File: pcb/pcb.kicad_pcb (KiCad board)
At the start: 4 copper layers, 32 x 39 mm, 88 parts, among them U1 JM20330, U2 SM2258XT, U3 FlashBGA152, U4 Conn_41PIN, U5 SY8008, U6 SY8008, U7 TX4314, Y1 25MHz, Y2 50MHz

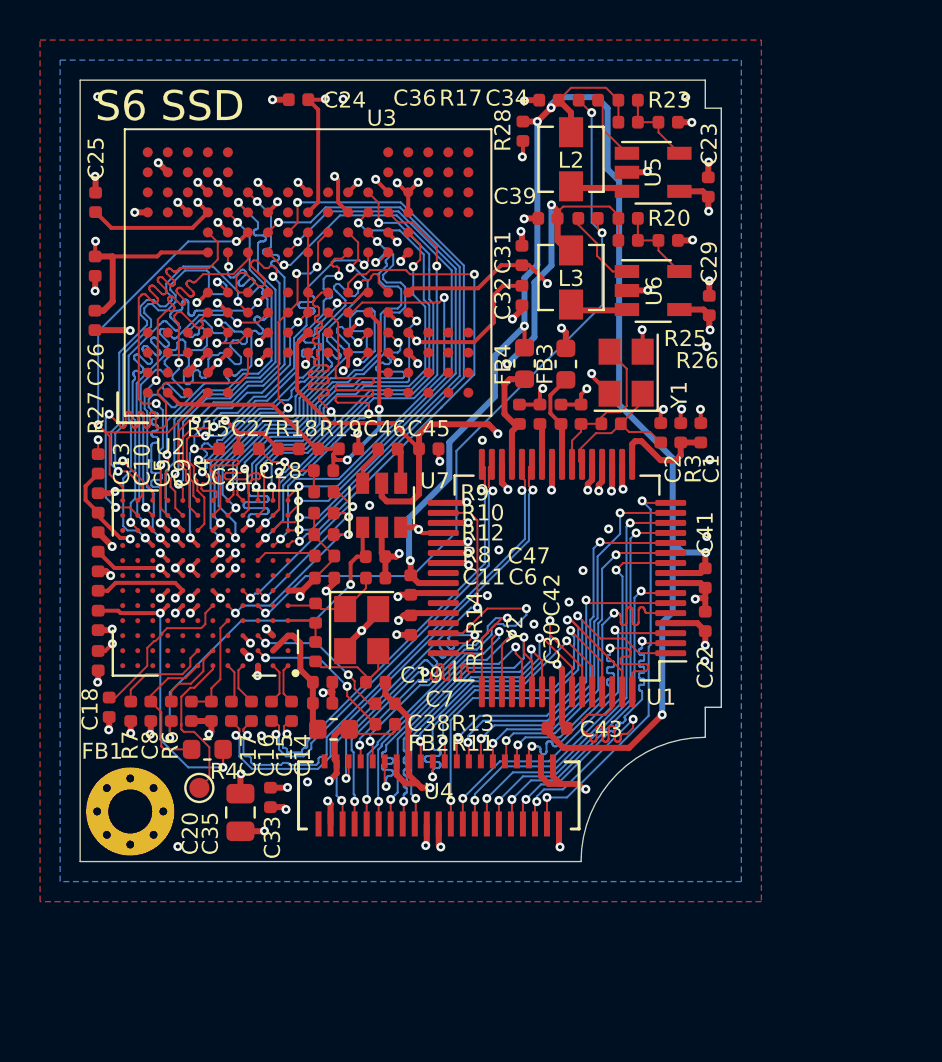
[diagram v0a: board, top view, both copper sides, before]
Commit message: Upgrade to 5.99, clean up
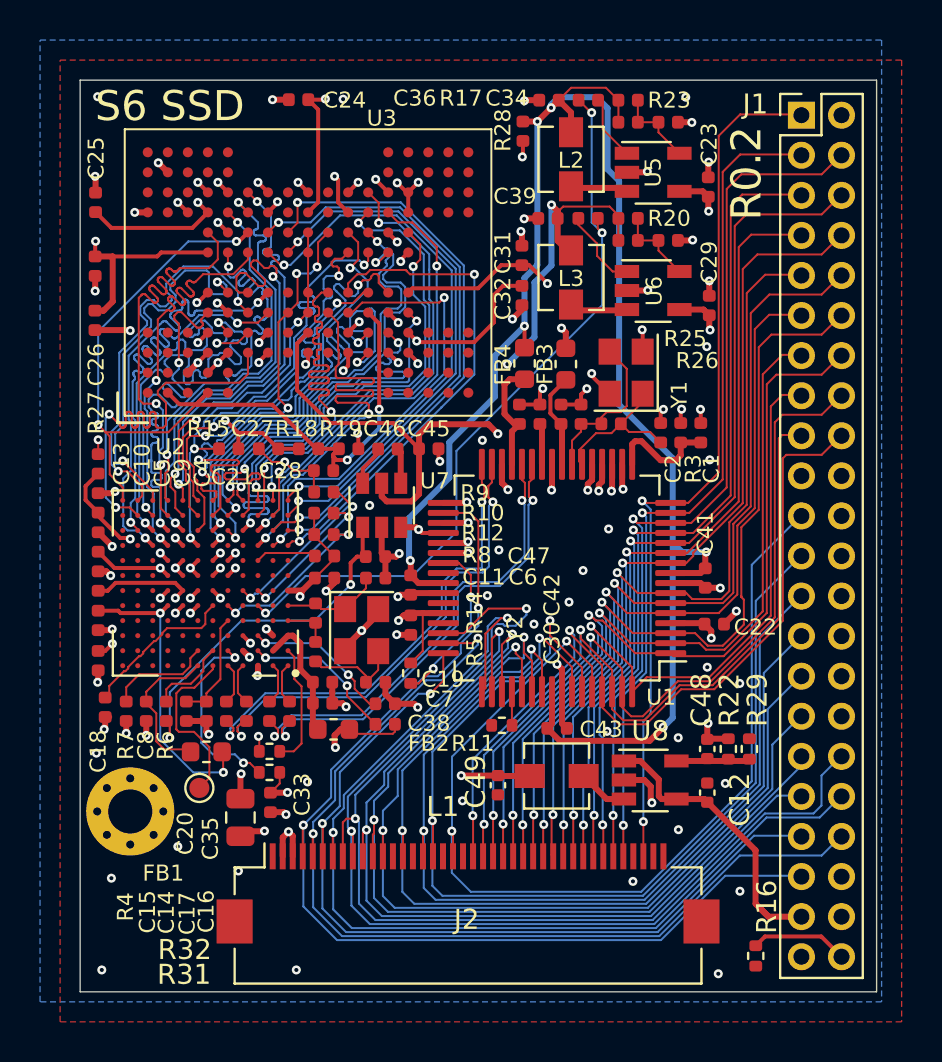
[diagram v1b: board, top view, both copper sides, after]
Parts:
- removed U4: Conn_41PIN, Footprints:FH35C-41S-0.3SHW
- added C12: 470nF, Capacitor_SMD:C_0402_1005Metric, F.Cu at (161.3, 126.6)
- added C48: 22pF, Capacitor_SMD:C_0402_1005Metric, F.Cu at (161.3, 124.4)
- added C49: 4.7uF, Capacitor_SMD:C_0402_1005Metric, F.Cu at (150.8, 126.2)
- added J1: Conn_02x22_Odd_Even, Connector_PinHeader_2.00mm:PinHeader_2x22_P2.00mm_Vertical, F.Cu at (166.0, 92.8)
- added J2: Conn_01x40_MountingPin, Connector_FFC-FPC:Hirose_FH12-40S-0.5SH_1x40-1MP_P0.50mm_Horizontal, F.Cu at (149.4, 131.6)
- added L1: 2.2uH, Inductor_SMD:L_Vishay_IHLP-1212, F.Cu at (153.8, 125.7)
- added R16: 10K, Resistor_SMD:R_0402_1005Metric, F.Cu at (163.7, 134.7)
- added R21: 10K, Resistor_SMD:R_0402_1005Metric, F.Cu at (151.1, 123.2)
- added R22: 46.4K, Resistor_SMD:R_0402_1005Metric, F.Cu at (162.3, 124.4)
- added R29: 10K, Resistor_SMD:R_0402_1005Metric, F.Cu at (163.4, 124.4)
- added R30: 10K, Resistor_SMD:R_0402_1005Metric, F.Cu at (146.5, 120.6)
- added R31: 10K, Resistor_SMD:R_0402_1005Metric, F.Cu at (139.4, 125.5)
- added R32: 200/1%, Resistor_SMD:R_0402_1005Metric, F.Cu at (139.4, 124.5)
- added U8: SY8008, Package_TO_SOT_SMD:TSOT-23-5, F.Cu at (158.4, 125.9)
- R12: value 10K -> NC
- R7: value 10K -> 0
- moved C14 2.25 mm to (138.3, 122.5)
- moved C15 2.25 mm to (137.3, 122.5)
- moved C16 1.90 mm to (140.4, 122.5)
- moved C17 1.90 mm to (139.4, 122.5)
- moved C22 0.47 mm to (161.7, 118.2), turned to 180 degrees
- moved C20 0.25 mm to (135.3, 122.5)
- moved C33 0.25 mm to (139.5, 127.0)
- moved C35 0.25 mm to (138.0, 127.8)
- moved R4 0.25 mm to (136.3, 122.5)
- moved R6 0.25 mm to (134.3, 122.5)
- moved C8 0.22 mm to (133.3, 122.5)
- moved R7 0.22 mm to (132.3, 122.5)
- moved C18 0.20 mm to (131.2, 122.3)
- moved FB1 0.13 mm to (136.3, 124.5)
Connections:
- U1 pad 27: Net-(C17-Pad1) -> Net-(C16-Pad1)
- U1 pad 28: Net-(C16-Pad1) -> Net-(C17-Pad1)
- U1 pad 31: Net-(C15-Pad1) -> Net-(C14-Pad1)
- U1 pad 32: Net-(C14-Pad1) -> Net-(C15-Pad1)
- U1 pad 39: GND -> Net-(R30-Pad2)
- U1 pad 40: (no net) -> unconnected-(U1-Pad40)
- U1 pad 43: (no net) -> unconnected-(U1-Pad43)
- U1 pad 45: (no net) -> unconnected-(U1-Pad45)
- U1 pad 52: (no net) -> Net-(R21-Pad1)
- U2 pad A1: Net-(C14-Pad2) -> Net-(C16-Pad2)
- U2 pad A10: (no net) -> unconnected-(U2-PadA10)
- U2 pad A11: (no net) -> unconnected-(U2-PadA11)
- U2 pad A12: (no net) -> unconnected-(U2-PadA12)
- U2 pad A2: Net-(C15-Pad2) -> Net-(C17-Pad2)
- U2 pad A4: Net-(C16-Pad2) -> Net-(C14-Pad2)
- U2 pad A5: Net-(C17-Pad2) -> Net-(C15-Pad2)
- U2 pad A8: (no net) -> unconnected-(U2-PadA8)
- U2 pad A9: (no net) -> unconnected-(U2-PadA9)
- U2 pad B1: (no net) -> Net-(R32-Pad1)
- U2 pad B10: (no net) -> unconnected-(U2-PadB10)
- U2 pad B11: (no net) -> unconnected-(U2-PadB11)
- U2 pad B12: (no net) -> unconnected-(U2-PadB12)
- U2 pad B5: (no net) -> Net-(R31-Pad1)
- U2 pad B8: (no net) -> unconnected-(U2-PadB8)
- U2 pad B9: (no net) -> unconnected-(U2-PadB9)
- U2 pad C10: (no net) -> unconnected-(U2-PadC10)
- U2 pad C11: (no net) -> unconnected-(U2-PadC11)
- U2 pad C12: (no net) -> unconnected-(U2-PadC12)
- U2 pad C5: (no net) -> unconnected-(U2-PadC5)
- U2 pad C6: (no net) -> unconnected-(U2-PadC6)
- U2 pad C7: (no net) -> unconnected-(U2-PadC7)
- U2 pad C8: (no net) -> unconnected-(U2-PadC8)
- U2 pad C9: (no net) -> unconnected-(U2-PadC9)
- U2 pad D10: (no net) -> unconnected-(U2-PadD10)
- U2 pad D11: (no net) -> unconnected-(U2-PadD11)
- U2 pad D12: (no net) -> unconnected-(U2-PadD12)
- U2 pad D2: (no net) -> unconnected-(U2-PadD2)
- U2 pad D3: (no net) -> unconnected-(U2-PadD3)
- U2 pad D4: (no net) -> unconnected-(U2-PadD4)
- U2 pad D6: (no net) -> unconnected-(U2-PadD6)
- U2 pad D7: (no net) -> unconnected-(U2-PadD7)
- U2 pad D8: (no net) -> unconnected-(U2-PadD8)
- U2 pad D9: (no net) -> unconnected-(U2-PadD9)
- U2 pad E10: (no net) -> unconnected-(U2-PadE10)
- U2 pad E11: (no net) -> unconnected-(U2-PadE11)
- U2 pad E12: (no net) -> unconnected-(U2-PadE12)
- U2 pad E2: (no net) -> unconnected-(U2-PadE2)
- U2 pad E4: (no net) -> unconnected-(U2-PadE4)
- U2 pad F10: (no net) -> unconnected-(U2-PadF10)
- U2 pad F11: (no net) -> unconnected-(U2-PadF11)
- U2 pad F12: (no net) -> unconnected-(U2-PadF12)
- U2 pad F2: (no net) -> unconnected-(U2-PadF2)
- U2 pad F5: (no net) -> unconnected-(U2-PadF5)
- U2 pad G1: (no net) -> unconnected-(U2-PadG1)
- U2 pad G10: (no net) -> unconnected-(U2-PadG10)
- U2 pad G11: (no net) -> unconnected-(U2-PadG11)
- U2 pad G12: (no net) -> unconnected-(U2-PadG12)
- U2 pad G2: (no net) -> unconnected-(U2-PadG2)
- U2 pad G3: (no net) -> unconnected-(U2-PadG3)
- U2 pad G4: (no net) -> unconnected-(U2-PadG4)
- U2 pad H1: (no net) -> unconnected-(U2-PadH1)
- U2 pad H10: (no net) -> unconnected-(U2-PadH10)
- U2 pad H11: (no net) -> unconnected-(U2-PadH11)
- U2 pad H12: (no net) -> unconnected-(U2-PadH12)
- U2 pad H2: (no net) -> unconnected-(U2-PadH2)
- U2 pad H4: (no net) -> unconnected-(U2-PadH4)
- U2 pad J11: (no net) -> unconnected-(U2-PadJ11)
- U2 pad J12: (no net) -> unconnected-(U2-PadJ12)
- U2 pad J4: (no net) -> unconnected-(U2-PadJ4)
- U2 pad J5: (no net) -> unconnected-(U2-PadJ5)
- U2 pad K12: (no net) -> unconnected-(U2-PadK12)
- U2 pad L12: (no net) -> unconnected-(U2-PadL12)
- U3 pad A1: Net-(U3-PadA1) -> unconnected-(U3-PadA1)
- U3 pad A11: Net-(U3-PadA11) -> unconnected-(U3-PadA11)
- U3 pad A12: Net-(U3-PadA12) -> unconnected-(U3-PadA12)
- U3 pad A13: Net-(U3-PadA13) -> unconnected-(U3-PadA13)
- U3 pad A2: Net-(U3-PadA2) -> unconnected-(U3-PadA2)
- U3 pad A3: Net-(U3-PadA3) -> unconnected-(U3-PadA3)
- U3 pad A4: Net-(U3-PadA4) -> unconnected-(U3-PadA4)
- U3 pad B10: Net-(U3-PadB10) -> unconnected-(U3-PadB10)
- U3 pad B11: Net-(U3-PadB11) -> unconnected-(U3-PadB11)
- U3 pad B13: Net-(U3-PadB13) -> unconnected-(U3-PadB13)
- U3 pad B2: Net-(U3-PadB2) -> unconnected-(U3-PadB2)
- U3 pad B3: Net-(U3-PadB3) -> unconnected-(U3-PadB3)
- U3 pad B4: Net-(U3-PadB4) -> unconnected-(U3-PadB4)
- U3 pad C1: Net-(U3-PadC1) -> unconnected-(U3-PadC1)
- U3 pad C11: Net-(U3-PadC11) -> unconnected-(U3-PadC11)
- U3 pad C12: Net-(U3-PadC12) -> unconnected-(U3-PadC12)
- U3 pad C13: Net-(U3-PadC13) -> unconnected-(U3-PadC13)
- U3 pad C3: Net-(U3-PadC3) -> unconnected-(U3-PadC3)
- U3 pad C4: Net-(U3-PadC4) -> unconnected-(U3-PadC4)
- U3 pad D12: Net-(U3-PadD12) -> unconnected-(U3-PadD12)
- U3 pad D13: Net-(U3-PadD13) -> unconnected-(U3-PadD13)
- U3 pad E1: Net-(U3-PadE1) -> unconnected-(U3-PadE1)
- U3 pad E12: Net-(U3-PadE12) -> unconnected-(U3-PadE12)
- U3 pad E13: Net-(U3-PadE13) -> unconnected-(U3-PadE13)
- U3 pad E2: Net-(U3-PadE2) -> unconnected-(U3-PadE2)
- U3 pad H10: Net-(U3-PadH10) -> unconnected-(U3-PadH10)
- U3 pad H11: Net-(U3-PadH11) -> unconnected-(U3-PadH11)
- U3 pad H3: Net-(U3-PadH3) -> unconnected-(U3-PadH3)
- U3 pad H4: Net-(U3-PadH4) -> unconnected-(U3-PadH4)
- U3 pad H6: Net-(U3-PadH6) -> unconnected-(U3-PadH6)
- U3 pad K10: Net-(U3-PadK10) -> unconnected-(U3-PadK10)
- U3 pad K11: Net-(U3-PadK11) -> unconnected-(U3-PadK11)
- U3 pad K3: Net-(U3-PadK3) -> unconnected-(U3-PadK3)
- U3 pad K4: Net-(U3-PadK4) -> unconnected-(U3-PadK4)
- U3 pad K8: Net-(U3-PadK8) -> unconnected-(U3-PadK8)
- U3 pad N1: Net-(U3-PadN1) -> unconnected-(U3-PadN1)
- U3 pad N12: Net-(U3-PadN12) -> unconnected-(U3-PadN12)
- U3 pad N13: Net-(U3-PadN13) -> unconnected-(U3-PadN13)
- U3 pad N2: Net-(U3-PadN2) -> unconnected-(U3-PadN2)
- U3 pad R1: Net-(U3-PadR1) -> unconnected-(U3-PadR1)
- U3 pad R10: Net-(U3-PadR10) -> unconnected-(U3-PadR10)
- U3 pad R11: Net-(U3-PadR11) -> unconnected-(U3-PadR11)
- U3 pad R12: Net-(U3-PadR12) -> unconnected-(U3-PadR12)
- U3 pad R13: Net-(U3-PadR13) -> unconnected-(U3-PadR13)
- U3 pad R2: Net-(U3-PadR2) -> unconnected-(U3-PadR2)
- U3 pad R3: Net-(U3-PadR3) -> unconnected-(U3-PadR3)
- U3 pad R4: Net-(U3-PadR4) -> unconnected-(U3-PadR4)
- U3 pad T1: Net-(U3-PadT1) -> unconnected-(U3-PadT1)
- U3 pad T10: Net-(U3-PadT10) -> unconnected-(U3-PadT10)
- U3 pad T11: Net-(U3-PadT11) -> unconnected-(U3-PadT11)
- U3 pad T12: Net-(U3-PadT12) -> unconnected-(U3-PadT12)
- U3 pad T13: Net-(U3-PadT13) -> unconnected-(U3-PadT13)
- U3 pad T2: Net-(U3-PadT2) -> unconnected-(U3-PadT2)
- U3 pad T3: Net-(U3-PadT3) -> unconnected-(U3-PadT3)
- U3 pad T4: Net-(U3-PadT4) -> unconnected-(U3-PadT4)
- U3 pad U1: Net-(U3-PadU1) -> unconnected-(U3-PadU1)
- U3 pad U10: Net-(U3-PadU10) -> unconnected-(U3-PadU10)
- U3 pad U11: Net-(U3-PadU11) -> unconnected-(U3-PadU11)
- U3 pad U12: Net-(U3-PadU12) -> unconnected-(U3-PadU12)
- U3 pad U13: Net-(U3-PadU13) -> unconnected-(U3-PadU13)
- U3 pad U2: Net-(U3-PadU2) -> unconnected-(U3-PadU2)
- U3 pad U3: Net-(U3-PadU3) -> unconnected-(U3-PadU3)
- U3 pad U4: Net-(U3-PadU4) -> unconnected-(U3-PadU4)
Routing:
- net /IDE_IOW: track 15.4 -> 53.2 mm
- net /IDE_PDIAG: track 16.9 -> 54.4 mm
- net /IDE_A2: track 15.6 -> 52.6 mm
- net /IDE_DMARQ: track 16.7 -> 50.2 mm
- net /IDE_DASP: track 20.2 -> 53.6 mm
- net /IDE_CS1: track 16.0 -> 49.3 mm
- net /IDE_IOR: track 16.9 -> 49.9 mm
- net /IDE_DMACK: track 16.3 -> 48.7 mm
- net /IDE_IORDY: track 15.9 -> 48.0 mm
- net /IDE_A0: track 16.0 -> 47.2 mm
- net /IDE_INTRQ: track 15.9 -> 46.7 mm
- net /IDE_A1: track 16.0 -> 46.4 mm
- net /IDE_D15: track 15.3 -> 41.0 mm
- net /IDE_CS0: track 18.0 -> 43.6 mm
- net /IDE_D12: track 17.2 -> 42.0 mm
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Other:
- board size 32 x 39 mm -> 39.8 x 45.5 mm
- net class Default removed
- rule pad_to_mask_clearance: 0.05 -> 0
- board text added: "R0.2"
- board text added: "S6 SSD Copyright 2021 W.Z."
- board text removed: "S6 SSD Copyright 2020 W.Z."

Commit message: Rev 0.3
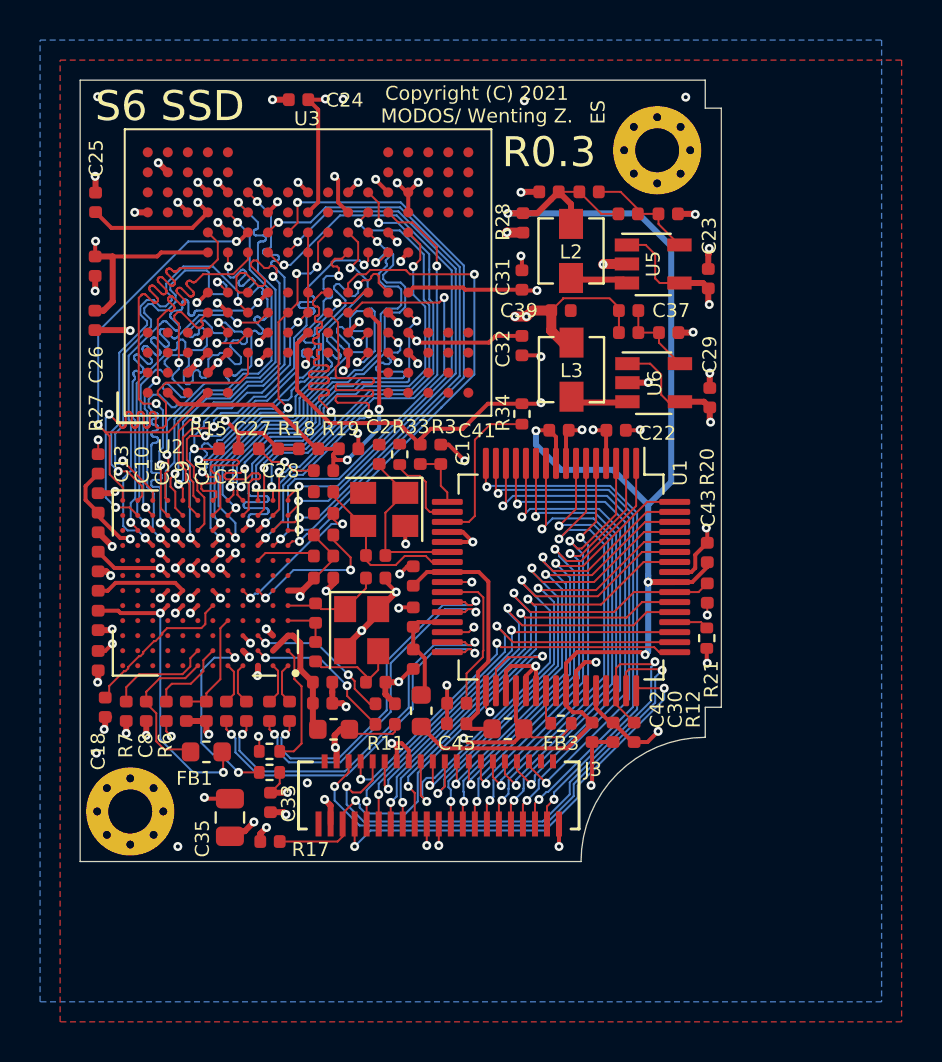
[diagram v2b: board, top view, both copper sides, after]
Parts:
- removed C12: 470nF, Capacitor_SMD:C_0402_1005Metric
- removed C47: 10uF, Capacitor_SMD:C_0402_1005Metric
- removed C48: 22pF, Capacitor_SMD:C_0402_1005Metric
- removed C49: 4.7uF, Capacitor_SMD:C_0402_1005Metric
- removed J1: Conn_02x22_Odd_Even, Connector_PinHeader_2.00mm:PinHeader_2x22_P2.00mm_Vertical
- removed J2: Conn_01x40_MountingPin, Connector_FFC-FPC:Hirose_FH12-40S-0.5SH_1x40-1MP_P0.50mm_Horizontal
- removed L1: 2.2uH, Inductor_SMD:L_Vishay_IHLP-1212
- removed R16, R29: 10K, Resistor_SMD:R_0402_1005Metric
- removed R22: 46.4K, Resistor_SMD:R_0402_1005Metric
- removed TP7: TestPoint, TestPoint:TestPoint_Pad_D1.0mm
- removed U7: TX4314, Package_TO_SOT_SMD:SOT-23-6
- removed U8: SY8008, Package_TO_SOT_SMD:TSOT-23-5
- added H2: MountingHole_Pad, MountingHole:MountingHole_2.2mm_M2_Pad_Via, F.Cu at (158.8, 94.5)
- added J3: S6, Footprints:FH35C-41S-0.3SHW, F.Cu at (147.9, 126.7)
- added R33: 0, Resistor_SMD:R_0402_1005Metric, F.Cu at (145.9, 109.7)
- added R34: 0, Resistor_SMD:R_0402_1005Metric, F.Cu at (152.1, 107.7)
- C31, C32, C33, C36, C38, C39: value 4.7uF -> 10uF
- H1: value MountingHole -> MountingHole_Pad
- R12, R13: value NC -> 10K
- R6: value 5.1K -> 2K
- moved R17 40.3 mm to (139.5, 129.0), turned to 0 degrees
- moved R20 19.6 mm to (161.3, 116.6), turned to 90 degrees
- moved FB3 18.4 mm to (151.3, 123.4), turned to 0 degrees
- moved R12 18.4 mm to (157.7, 123.5), turned to 90 degrees
- moved FB4 18.1 mm to (147.0, 122.5), turned to -90 degrees
- moved R1 15.0 mm to (148.8, 122.1), turned to 0 degrees
- moved C2 14.1 mm to (144.9, 109.7)
- moved Y1 13.9 mm to (145.2, 112.4), turned to 180 degrees
- moved C45 13.8 mm to (148.8, 123.1), turned to 0 degrees
- moved R2 13.5 mm to (144.8, 114.7)
- moved C3 13.4 mm to (142.2, 111.5), turned to 180 degrees
- moved R3 13.0 mm to (147.0, 109.7)
- moved C1 13.0 mm to (148.0, 109.7)
- moved C42 11.7 mm to (155.6, 123.5)
- moved C43 11.5 mm to (161.3, 114.6), turned to -90 degrees
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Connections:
- C45 pad 2: +3V3 -> Net-(C40-Pad2)
- C46 pad 1: Net-(C46-Pad1) -> GND
- C46 pad 2: Net-(C46-Pad2) -> Net-(C44-Pad2)
- H1 pad 1: (no net) -> GND
- R12 pad 1: /P24 -> +3V3
- R12 pad 2: +3V3 -> /IDE_PDIAG
- R17 pad 1: Net-(R17-Pad1) -> +3V3
- R17 pad 2: /P27 -> /IDE_DASP
- R20 pad 1: Net-(R20-Pad1) -> +3V3
- R20 pad 2: /P27 -> /IDE_IORDY
- R6 pad 2: +5V -> +3V3
- U1 pad 18: GND -> Net-(R33-Pad2)
- U1 pad 19: +3V3 -> Net-(R34-Pad2)
- U2 pad A6: /EXPWD -> unconnected-(U2-PadA6)
- U2 pad E3: /P27 -> unconnected-(U2-PadE3)
- U2 pad E5: /P24 -> unconnected-(U2-PadE5)
- U2 pad H9: GND -> +VCCFQ
- U5 pad 1: Net-(R17-Pad1) -> +3V3
- U6 pad 1: Net-(R20-Pad1) -> +3V3
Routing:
- net /P27: track 37.6 -> 0.00 mm, vias 3 -> 0
- net /IDE_A2: track 52.6 -> 19.9 mm
- net /IDE_DASP: track 53.6 -> 22.8 mm
- net /IDE_DMARQ: track 50.2 -> 22.0 mm
- net /IDE_IOW: track 53.2 -> 25.7 mm
- net /IDE_IOR: track 49.9 -> 22.5 mm
- net /IDE_DMACK: track 48.7 -> 21.5 mm
- net /IDE_A1: track 46.4 -> 20.6 mm
- net /IDE_PDIAG: track 54.4 -> 29.2 mm
- net /IDE_A0: track 47.2 -> 22.1 mm
- net /IDE_INTRQ: track 46.7 -> 22.5 mm
- net /IDE_CS1: track 49.3 -> 26.2 mm
- net /IDE_IORDY: track 48.0 -> 25.3 mm
- net /IDE_CS0: track 43.6 -> 22.0 mm
- net /IDE_D12: track 42.0 -> 21.3 mm
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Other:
- board size 39.8 x 45.5 mm -> 32 x 39 mm
- board text added: "Copyright (C) 2021 MODOS/ Wenting Z."
- board text added: "Copyright Wenting Zhang 2021 This device is Open Hardware and the design source is licensed under the CERN-OHL-P v2. You could download the source from github.com/zephray/ BenqS6-SSD."
- board text added: "ES"
- board text added: "GB"
- board text added: "Prototype Not For Sale"
- board text added: "R0.3"
- board text added: "SSD Upgrade For Benq S6"
- board text removed: "R0.2"
- board text removed: "S6 SSD Copyright 2021 W.Z."
